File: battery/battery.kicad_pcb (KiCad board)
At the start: 2 copper layers, 73.7 x 63.5 mm, 48 parts, among them J1 batt_1, J2 batt_2, J3 batt_3, J4 batt_4, J5 reed_switch, J6 toPcb+, J7 toPcb-, J8 on_signal, Q1 batt1_sw, Q2 batt2_sw, Q3 batt3_sw, Q4 batt4_sw, Q5 Q_NPN_CBE, U1 LM1117-5.0, U2 LTV-817S

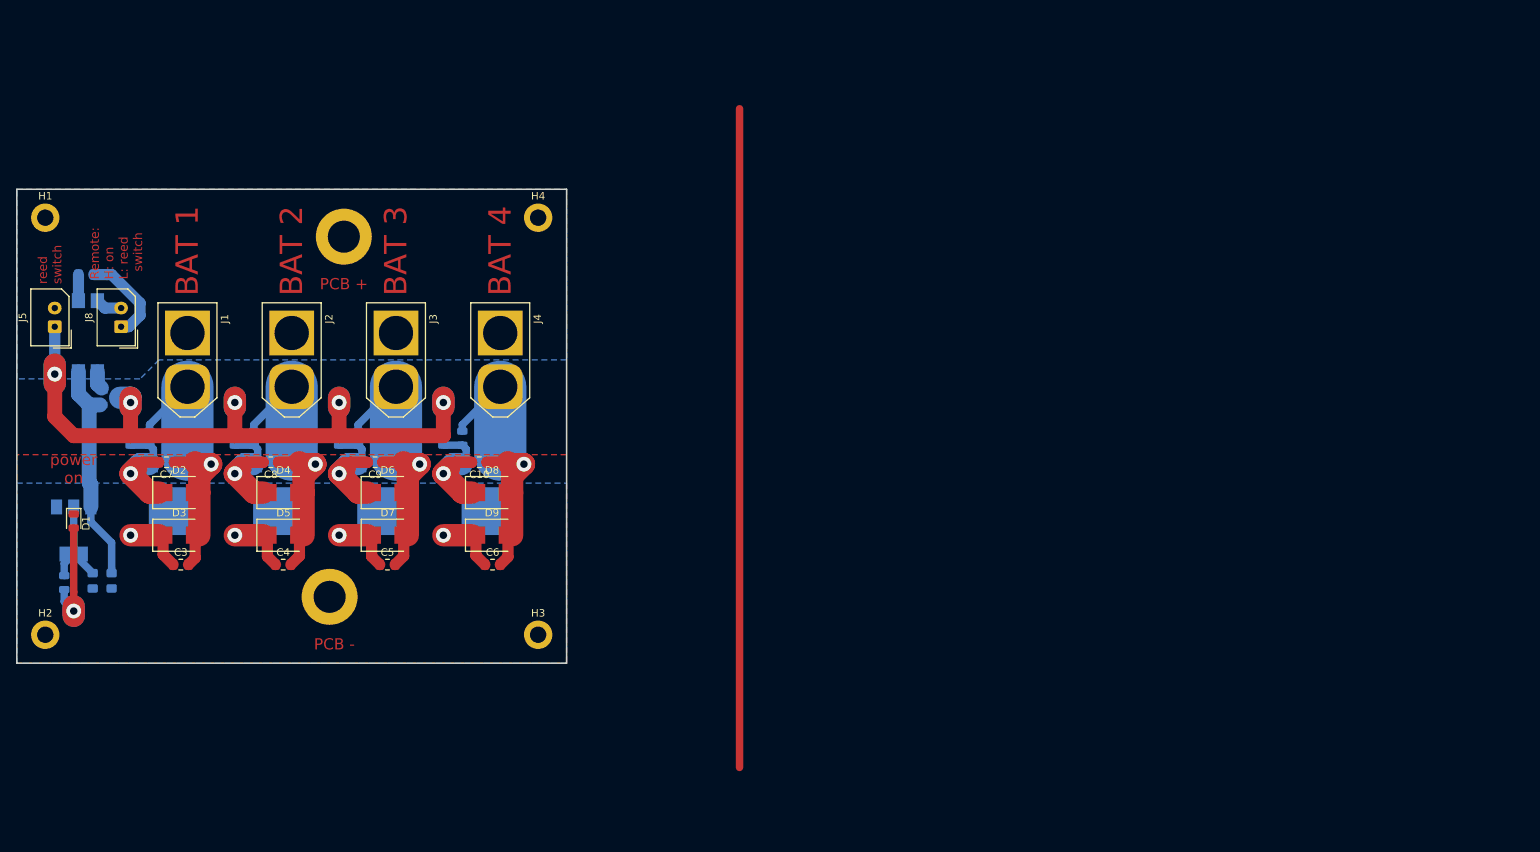
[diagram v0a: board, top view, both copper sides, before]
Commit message: fix
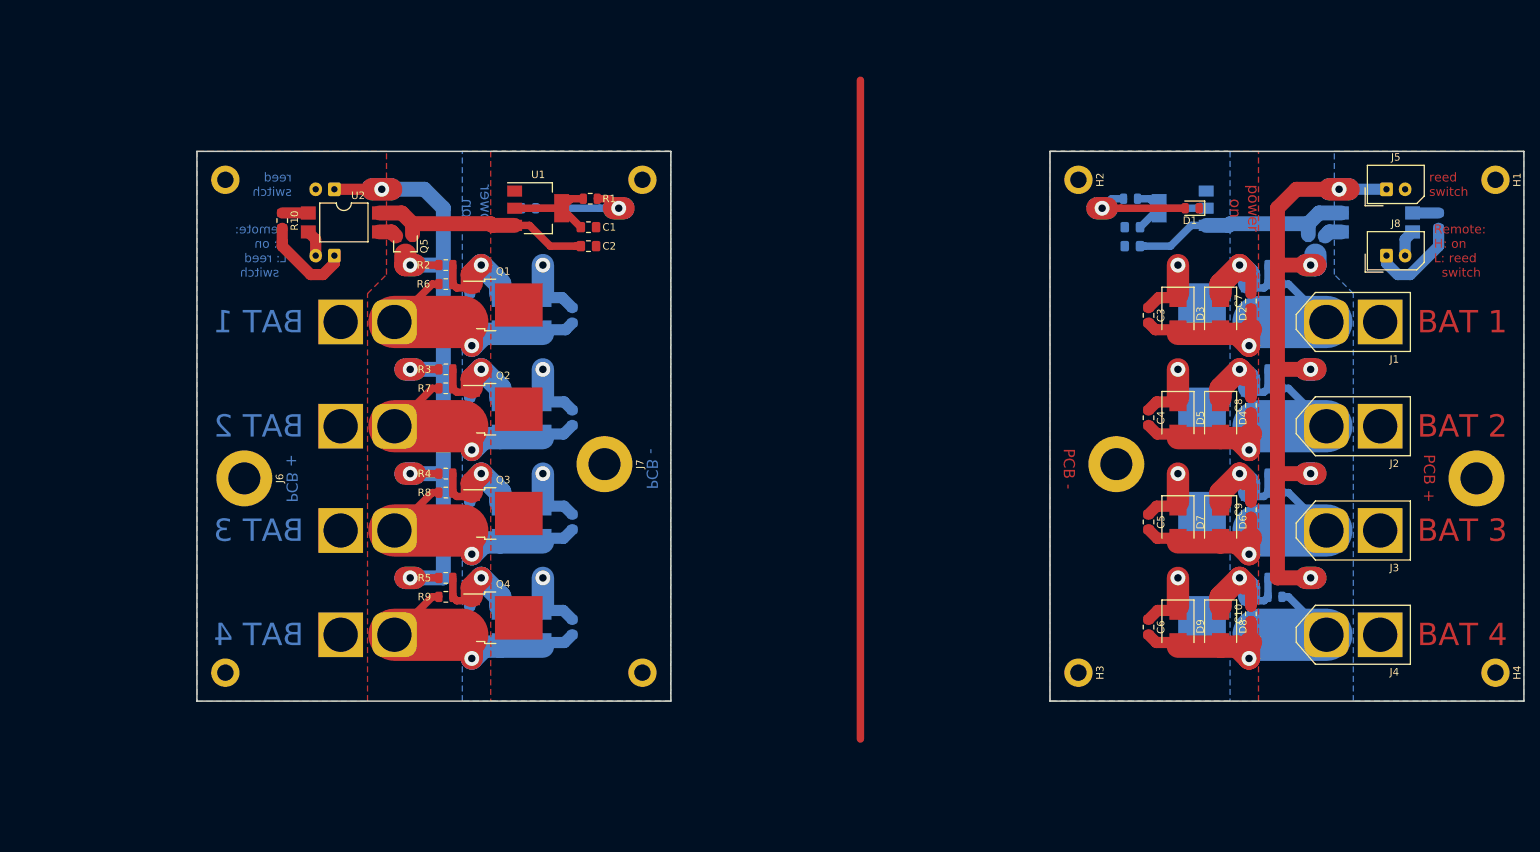
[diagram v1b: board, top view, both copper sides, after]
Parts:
- removed the C1 at (65.4, 116.0)
- removed the C10 at (117.2, 100.1)
- removed the C2 at (67.9, 116.0)
- removed the C3 at (77.2, 113.8)
- removed the C4 at (90.9, 113.8)
- removed the C5 at (104.9, 113.8)
- removed the C6 at (119.0, 113.8)
- removed the C7 at (75.3, 100.1)
- removed the C8 at (89.3, 100.1)
- removed the C9 at (103.2, 100.1)
- removed the D1 at (62.9, 108.0)
- removed the D2 at (77.0, 104.1)
- removed the D3 at (77.0, 109.9)
- removed the D4 at (91.0, 104.1)
- removed the D5 at (91.0, 109.9)
- removed the D6 at (104.9, 104.1)
- removed the D7 at (104.9, 109.9)
- removed the D8 at (118.9, 104.1)
- removed the D9 at (118.9, 109.9)
- removed the H1 at (59.1, 67.3)
- removed the H2 at (59.1, 123.2)
- removed the H3 at (125.1, 123.2)
- removed the H4 at (125.1, 67.3)
- removed the J1 at (78.1, 86.4)
- removed the J2 at (92.1, 86.4)
- removed the J3 at (106.0, 86.4)
- removed the J4 at (120.0, 86.4)
- removed the J5 at (60.3, 81.9)
- removed the J6 at (99.1, 69.8)
- removed the J7 at (97.2, 118.1)
- removed the J8 at (69.2, 81.9)
- removed the Q1 at (75.8, 104.5)
- removed the Q2 at (89.8, 104.5)
- removed the Q3 at (103.8, 104.5)
- removed the Q4 at (117.7, 104.5)
- removed the Q5 at (67.9, 91.4)
- removed the R1 at (61.6, 116.2)
- removed the R10 at (64.5, 74.9)
- removed the R2 at (70.5, 96.9)
- removed the R3 at (84.5, 96.9)
- removed the R4 at (98.4, 96.9)
- removed the R5 at (112.4, 96.9)
- removed the R6 at (73.0, 96.9)
- removed the R7 at (87.0, 96.9)
- removed the R8 at (101.0, 96.9)
- removed the R9 at (114.9, 96.9)
- removed the U1 at (62.9, 109.2)
- removed the U2 at (64.8, 83.2)
- added C1: C_Small, Capacitor_SMD:C_0805_2012Metric_Pad1.15x1.40mm_HandSolder, B.Cu at (204.7, 68.6)
- added C1: C_Small, Capacitor_SMD:C_0805_2012Metric_Pad1.15x1.40mm_HandSolder, F.Cu at (131.8, 68.6)
- added C10: 100n, Capacitor_SMD:C_0805_2012Metric_Pad1.15x1.40mm_HandSolder, F.Cu at (220.6, 120.4)
- added C10: 100n, Capacitor_SMD:C_0805_2012Metric_Pad1.15x1.40mm_HandSolder, B.Cu at (116.0, 120.4)
- added C2: C_Small, Capacitor_SMD:C_0805_2012Metric_Pad1.15x1.40mm_HandSolder, B.Cu at (204.7, 71.1)
- added C2: C_Small, Capacitor_SMD:C_0805_2012Metric_Pad1.15x1.40mm_HandSolder, F.Cu at (131.8, 71.1)
- added C3: 10uF, Capacitor_SMD:C_0805_2012Metric_Pad1.15x1.40mm_HandSolder, F.Cu at (206.9, 80.4)
- added C3: 10uF, Capacitor_SMD:C_0805_2012Metric_Pad1.15x1.40mm_HandSolder, B.Cu at (129.7, 80.4)
- added C4: 10uF, Capacitor_SMD:C_0805_2012Metric_Pad1.15x1.40mm_HandSolder, F.Cu at (206.9, 94.1)
- added C4: 10uF, Capacitor_SMD:C_0805_2012Metric_Pad1.15x1.40mm_HandSolder, B.Cu at (129.7, 94.1)
- added C5: 10uF, Capacitor_SMD:C_0805_2012Metric_Pad1.15x1.40mm_HandSolder, F.Cu at (206.9, 108.1)
- added C5: 10uF, Capacitor_SMD:C_0805_2012Metric_Pad1.15x1.40mm_HandSolder, B.Cu at (129.7, 108.1)
- added C6: 10uF, Capacitor_SMD:C_0805_2012Metric_Pad1.15x1.40mm_HandSolder, F.Cu at (206.9, 122.2)
- added C6: 10uF, Capacitor_SMD:C_0805_2012Metric_Pad1.15x1.40mm_HandSolder, B.Cu at (129.7, 122.2)
- added C7: 100n, Capacitor_SMD:C_0805_2012Metric_Pad1.15x1.40mm_HandSolder, F.Cu at (220.6, 78.5)
- added C7: 100n, Capacitor_SMD:C_0805_2012Metric_Pad1.15x1.40mm_HandSolder, B.Cu at (116.0, 78.5)
- added C8: 100n, Capacitor_SMD:C_0805_2012Metric_Pad1.15x1.40mm_HandSolder, F.Cu at (220.6, 92.4)
- added C8: 100n, Capacitor_SMD:C_0805_2012Metric_Pad1.15x1.40mm_HandSolder, B.Cu at (116.0, 92.4)
- added C9: 100n, Capacitor_SMD:C_0805_2012Metric_Pad1.15x1.40mm_HandSolder, F.Cu at (220.6, 106.4)
- added C9: 100n, Capacitor_SMD:C_0805_2012Metric_Pad1.15x1.40mm_HandSolder, B.Cu at (116.0, 106.4)
- added D1: power_ok, LED_SMD:LED_0805_2012Metric, F.Cu at (212.7, 66.0)
- added D1: power_ok, LED_SMD:LED_0805_2012Metric, B.Cu at (123.8, 66.0)
- added D2: D_TVS, Diode_SMD:D_SMB, F.Cu at (216.5, 80.2)
- added D2: D_TVS, Diode_SMD:D_SMB, B.Cu at (120.0, 80.2)
- added D3: D_TVS, Diode_SMD:D_SMB, F.Cu at (210.8, 80.2)
- added D3: D_TVS, Diode_SMD:D_SMB, B.Cu at (125.7, 80.2)
- added D4: D_TVS, Diode_SMD:D_SMB, F.Cu at (216.5, 94.1)
- added D4: D_TVS, Diode_SMD:D_SMB, B.Cu at (120.0, 94.1)
- added D5: D_TVS, Diode_SMD:D_SMB, F.Cu at (210.8, 94.1)
- added D5: D_TVS, Diode_SMD:D_SMB, B.Cu at (125.7, 94.1)
- added D6: D_TVS, Diode_SMD:D_SMB, F.Cu at (216.5, 108.1)
- added D6: D_TVS, Diode_SMD:D_SMB, B.Cu at (120.0, 108.1)
- added D7: D_TVS, Diode_SMD:D_SMB, F.Cu at (210.8, 108.1)
- added D7: D_TVS, Diode_SMD:D_SMB, B.Cu at (125.7, 108.1)
- added D8: D_TVS, Diode_SMD:D_SMB, F.Cu at (216.5, 122.1)
- added D8: D_TVS, Diode_SMD:D_SMB, B.Cu at (120.0, 122.1)
- added D9: D_TVS, Diode_SMD:D_SMB, F.Cu at (210.8, 122.1)
- added D9: D_TVS, Diode_SMD:D_SMB, B.Cu at (125.7, 122.1)
- added H1: mnt, MountingHole:MountingHole_2.2mm_M2_DIN965_Pad, F.Cu at (253.4, 62.2)
- added H1: mnt, MountingHole:MountingHole_2.2mm_M2_DIN965_Pad, B.Cu at (83.2, 62.2)
- added H2: mnt, MountingHole:MountingHole_2.2mm_M2_DIN965_Pad, F.Cu at (197.5, 62.2)
- added H2: mnt, MountingHole:MountingHole_2.2mm_M2_DIN965_Pad, B.Cu at (139.1, 62.2)
- added H3: mnt, MountingHole:MountingHole_2.2mm_M2_DIN965_Pad, F.Cu at (197.5, 128.3)
- added H3: mnt, MountingHole:MountingHole_2.2mm_M2_DIN965_Pad, B.Cu at (139.1, 128.3)
- added H4: mnt, MountingHole:MountingHole_2.2mm_M2_DIN965_Pad, F.Cu at (253.4, 128.3)
- added H4: mnt, MountingHole:MountingHole_2.2mm_M2_DIN965_Pad, B.Cu at (83.2, 128.3)
- added J1: batt_1, power_connectors:XT60UPB-M, F.Cu at (234.3, 81.3)
- added J1: batt_1, power_connectors:XT60UPB-M, B.Cu at (102.2, 81.3)
- added J2: batt_2, power_connectors:XT60UPB-M, F.Cu at (234.3, 95.2)
- added J2: batt_2, power_connectors:XT60UPB-M, B.Cu at (102.2, 95.2)
- added J3: batt_3, power_connectors:XT60UPB-M, F.Cu at (234.3, 109.2)
- added J3: batt_3, power_connectors:XT60UPB-M, B.Cu at (102.2, 109.2)
- added J4: batt_4, power_connectors:XT60UPB-M, F.Cu at (234.3, 123.2)
- added J4: batt_4, power_connectors:XT60UPB-M, B.Cu at (102.2, 123.2)
- added J5: reed_switch, Connector_Molex:Molex_SPOX_5267-02A_1x02_P2.50mm_Vertical, F.Cu at (238.8, 63.5)
- added J5: reed_switch, Connector_Molex:Molex_SPOX_5267-02A_1x02_P2.50mm_Vertical, B.Cu at (97.8, 63.5)
- added J6: toPcb+, MountingHole:MountingHole_4.3mm_M4_DIN965_Pad, B.Cu at (250.8, 102.2)
- added J6: toPcb+, MountingHole:MountingHole_4.3mm_M4_DIN965_Pad, F.Cu at (85.7, 102.2)
- added J7: toPcb-, MountingHole:MountingHole_4.3mm_M4_DIN965_Pad, B.Cu at (202.6, 100.3)
- added J7: toPcb-, MountingHole:MountingHole_4.3mm_M4_DIN965_Pad, F.Cu at (134.0, 100.3)
- added J8: on_signal, Connector_Molex:Molex_SPOX_5267-02A_1x02_P2.50mm_Vertical, F.Cu at (238.8, 72.4)
- added J8: on_signal, Connector_Molex:Molex_SPOX_5267-02A_1x02_P2.50mm_Vertical, B.Cu at (97.8, 72.4)
- added Q1: batt1_sw, Package_TO_SOT_SMD:TO-252-2, B.Cu at (216.1, 79.0)
- added Q1: batt1_sw, Package_TO_SOT_SMD:TO-252-2, F.Cu at (120.4, 79.0)
- added Q2: batt2_sw, Package_TO_SOT_SMD:TO-252-2, B.Cu at (216.1, 93.0)
- added Q2: batt2_sw, Package_TO_SOT_SMD:TO-252-2, F.Cu at (120.4, 93.0)
- added Q3: batt3_sw, Package_TO_SOT_SMD:TO-252-2, B.Cu at (216.1, 106.9)
- added Q3: batt3_sw, Package_TO_SOT_SMD:TO-252-2, F.Cu at (120.4, 106.9)
- added Q4: batt4_sw, Package_TO_SOT_SMD:TO-252-2, B.Cu at (216.1, 120.9)
- added Q4: batt4_sw, Package_TO_SOT_SMD:TO-252-2, F.Cu at (120.4, 120.9)
- added Q5: Q_NPN_CBE, Package_TO_SOT_SMD:SOT-23, B.Cu at (229.2, 71.1)
- added Q5: Q_NPN_CBE, Package_TO_SOT_SMD:SOT-23, F.Cu at (107.3, 71.1)
- added R1: 400, Resistor_SMD:R_0805_2012Metric, B.Cu at (204.5, 64.8)
- added R1: 400, Resistor_SMD:R_0805_2012Metric, F.Cu at (132.1, 64.8)
- added R10: R, Resistor_SMD:R_0805_2012Metric_Pad1.15x1.40mm_HandSolder, B.Cu at (245.7, 67.7)
- added R10: R, Resistor_SMD:R_0805_2012Metric_Pad1.15x1.40mm_HandSolder, F.Cu at (90.8, 67.7)
- added R2: 100, Resistor_SMD:R_0805_2012Metric, B.Cu at (223.8, 73.7)
- added R2: 100, Resistor_SMD:R_0805_2012Metric, F.Cu at (112.7, 73.7)
- added R3: 100, Resistor_SMD:R_0805_2012Metric, B.Cu at (223.8, 87.6)
- added R3: 100, Resistor_SMD:R_0805_2012Metric, F.Cu at (112.7, 87.6)
- added R4: 100, Resistor_SMD:R_0805_2012Metric, B.Cu at (223.8, 101.6)
- added R4: 100, Resistor_SMD:R_0805_2012Metric, F.Cu at (112.7, 101.6)
- added R5: 100, Resistor_SMD:R_0805_2012Metric, B.Cu at (223.8, 115.6)
- added R5: 100, Resistor_SMD:R_0805_2012Metric, F.Cu at (112.7, 115.6)
- added R6: 47k, Resistor_SMD:R_0805_2012Metric, B.Cu at (223.8, 76.2)
- added R6: 47k, Resistor_SMD:R_0805_2012Metric, F.Cu at (112.7, 76.2)
- added R7: 47k, Resistor_SMD:R_0805_2012Metric, B.Cu at (223.8, 90.2)
- added R7: 47k, Resistor_SMD:R_0805_2012Metric, F.Cu at (112.7, 90.2)
- added R8: 47k, Resistor_SMD:R_0805_2012Metric, B.Cu at (223.8, 104.1)
- added R8: 47k, Resistor_SMD:R_0805_2012Metric, F.Cu at (112.7, 104.1)
- added R9: 47k, Resistor_SMD:R_0805_2012Metric, B.Cu at (223.8, 118.1)
- added R9: 47k, Resistor_SMD:R_0805_2012Metric, F.Cu at (112.7, 118.1)
- added U1: LM1117-5.0, Package_TO_SOT_SMD:SOT-223-3_TabPin2, B.Cu at (211.5, 66.0)
- added U1: LM1117-5.0, Package_TO_SOT_SMD:SOT-223-3_TabPin2, F.Cu at (125.1, 66.0)
- added U2: LTV-817S, Package_DIP:SMDIP-4_W9.53mm, B.Cu at (237.5, 67.9)
- added U2: LTV-817S, Package_DIP:SMDIP-4_W9.53mm, F.Cu at (99.1, 67.9)
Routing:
- net Net-(J5-Pad1): track 115.6 -> 231.2 mm, vias 5 -> 10
- net Net-(C5-Pad2): track 43.8 -> 87.6 mm, vias 1 -> 2
- net Net-(C4-Pad2): track 43.8 -> 87.6 mm, vias 1 -> 2
- net Net-(C10-Pad1): track 43.7 -> 87.5 mm, vias 1 -> 2
- net Net-(C3-Pad2): track 40.4 -> 80.8 mm, vias 1 -> 2
- net gnd: track 33.0 -> 65.9 mm, vias 4 -> 8
- net Vin: track 30.3 -> 60.6 mm
- net Net-(C8-Pad2): track 21.4 -> 42.7 mm, vias 1 -> 2
- net Net-(C9-Pad2): track 20.9 -> 41.7 mm, vias 1 -> 2
- net Net-(C10-Pad2): track 20.9 -> 41.7 mm, vias 1 -> 2
- net Net-(C7-Pad2): track 18.6 -> 37.2 mm, vias 1 -> 2
- net Net-(D1-Pad2): track 17.1 -> 34.1 mm, vias 1 -> 2
- net Net-(C1-Pad1): track 13.3 -> 26.7 mm
- net Net-(J8-Pad1): track 12.6 -> 25.2 mm
- net Net-(J8-Pad2): track 3.59 -> 7.17 mm
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- added copper zone on F.Cu, net Vin
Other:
- board size 73.7 x 63.5 mm -> 177.8 x 73.7 mm

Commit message: new schematic
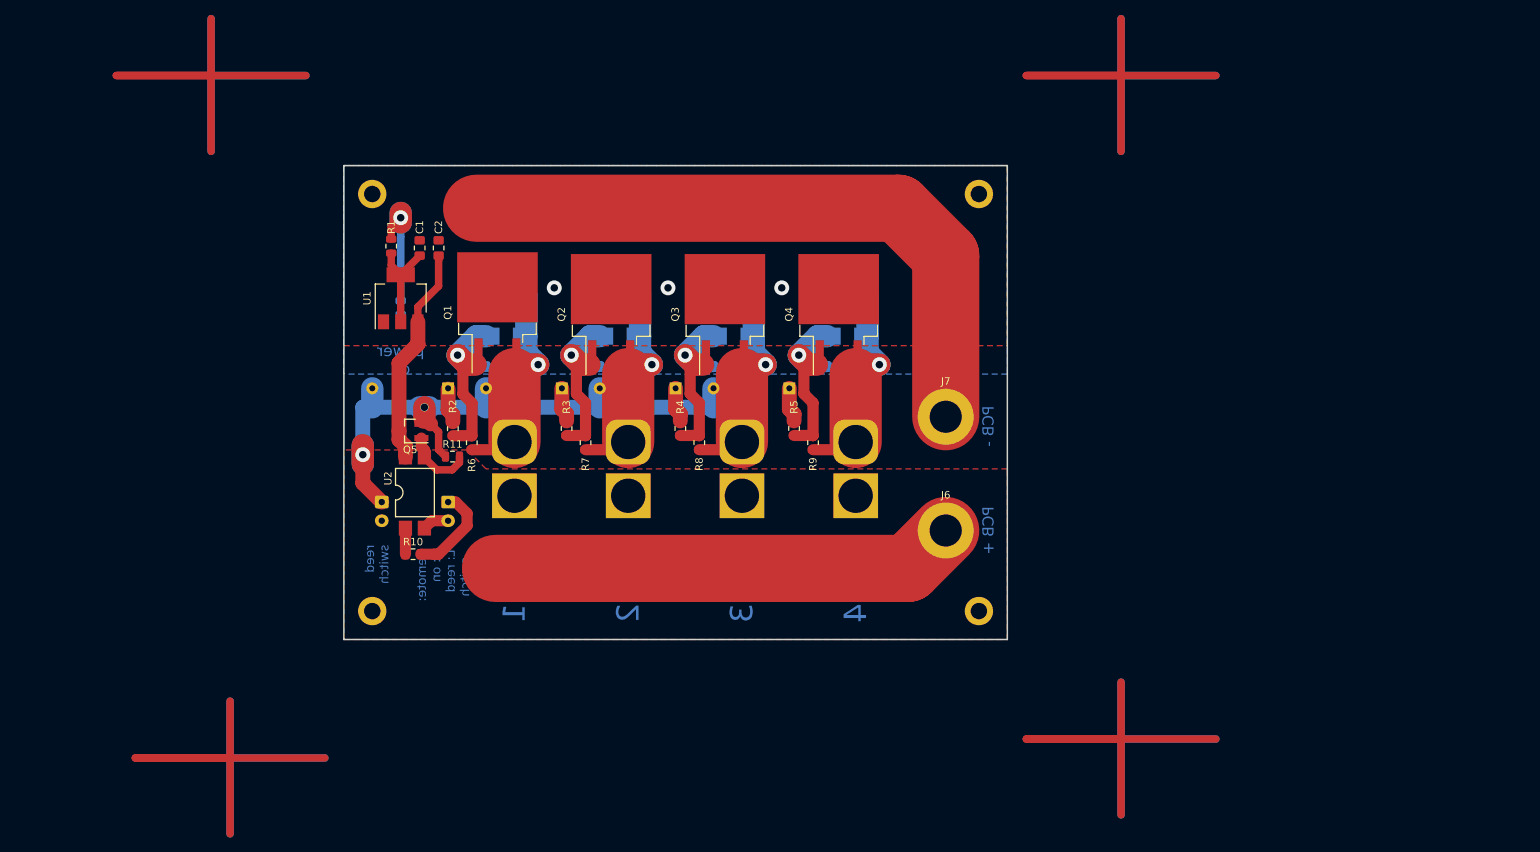
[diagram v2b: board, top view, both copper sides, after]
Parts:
- removed the C1 at (204.7, 68.6)
- removed the C10 at (220.6, 120.4)
- removed the C10 at (116.0, 120.4)
- removed the C2 at (204.7, 71.1)
- removed the C3 at (206.9, 80.4)
- removed the C3 at (129.7, 80.4)
- removed the C4 at (206.9, 94.1)
- removed the C4 at (129.7, 94.1)
- removed the C5 at (206.9, 108.1)
- removed the C5 at (129.7, 108.1)
- removed the C6 at (206.9, 122.2)
- removed the C6 at (129.7, 122.2)
- removed the C7 at (220.6, 78.5)
- removed the C8 at (220.6, 92.4)
- removed the C8 at (116.0, 92.4)
- removed the C9 at (220.6, 106.4)
- removed the C9 at (116.0, 106.4)
- removed the D1 at (212.7, 66.0)
- removed the D2 at (216.5, 80.2)
- removed the D3 at (210.8, 80.2)
- removed the D4 at (216.5, 94.1)
- removed the D4 at (120.0, 94.1)
- removed the D5 at (210.8, 94.1)
- removed the D5 at (125.7, 94.1)
- removed the D6 at (216.5, 108.1)
- removed the D6 at (120.0, 108.1)
- removed the D7 at (210.8, 108.1)
- removed the D7 at (125.7, 108.1)
- removed the D8 at (216.5, 122.1)
- removed the D8 at (120.0, 122.1)
- removed the D9 at (210.8, 122.1)
- removed the D9 at (125.7, 122.1)
- removed the H1 at (253.4, 62.2)
- removed the H2 at (197.5, 62.2)
- removed the H3 at (197.5, 128.3)
- removed the H3 at (139.1, 128.3)
- removed the H4 at (253.4, 128.3)
- removed the J1 at (234.3, 81.3)
- removed the J2 at (234.3, 95.2)
- removed the J2 at (102.2, 95.2)
- removed the J3 at (234.3, 109.2)
- removed the J3 at (102.2, 109.2)
- removed the J4 at (234.3, 123.2)
- removed the J4 at (102.2, 123.2)
- removed the J5 at (238.8, 63.5)
- removed the J6 at (250.8, 102.2)
- removed the J7 at (202.6, 100.3)
- removed the J8 at (238.8, 72.4)
- removed the Q1 at (216.1, 79.0)
- removed the Q1 at (120.4, 79.0)
- removed the Q2 at (216.1, 93.0)
- removed the Q2 at (120.4, 93.0)
- removed the Q3 at (216.1, 106.9)
- removed the Q3 at (120.4, 106.9)
- removed the Q4 at (216.1, 120.9)
- removed the Q4 at (120.4, 120.9)
- removed the Q5 at (229.2, 71.1)
- removed the Q5 at (107.3, 71.1)
- removed the R1 at (204.5, 64.8)
- removed the R10 at (245.7, 67.7)
- removed the R2 at (223.8, 73.7)
- removed the R3 at (223.8, 87.6)
- removed the R4 at (223.8, 101.6)
- removed the R4 at (112.7, 101.6)
- removed the R5 at (223.8, 115.6)
- removed the R5 at (112.7, 115.6)
- removed the R6 at (223.8, 76.2)
- removed the R7 at (223.8, 90.2)
- removed the R7 at (112.7, 90.2)
- removed the R8 at (223.8, 104.1)
- removed the R8 at (112.7, 104.1)
- removed the R9 at (223.8, 118.1)
- removed the R9 at (112.7, 118.1)
- removed the U1 at (211.5, 66.0)
- removed the U2 at (237.5, 67.9)
- added C10: 100n, Capacitor_SMD:C_0805_2012Metric_Pad1.15x1.40mm_HandSolder, B.Cu at (164.8, 87.2)
- added C3: 10uF, Capacitor_SMD:C_1206_3216Metric_Pad1.42x1.75mm_HandSolder, B.Cu at (121.0, 73.5)
- added C4: 10uF, Capacitor_SMD:C_1206_3216Metric_Pad1.42x1.75mm_HandSolder, B.Cu at (136.0, 73.5)
- added C5: 10uF, Capacitor_SMD:C_1206_3216Metric_Pad1.42x1.75mm_HandSolder, B.Cu at (151.3, 73.5)
- added C6: 10uF, Capacitor_SMD:C_1206_3216Metric_Pad1.42x1.75mm_HandSolder, B.Cu at (166.6, 73.5)
- added C8: 100n, Capacitor_SMD:C_0805_2012Metric_Pad1.15x1.40mm_HandSolder, B.Cu at (134.4, 87.2)
- added C9: 100n, Capacitor_SMD:C_0805_2012Metric_Pad1.15x1.40mm_HandSolder, B.Cu at (149.6, 87.2)
- added D10: bat48, Diode_THT:D_DO-35_SOD27_P10.16mm_Horizontal, B.Cu at (113.0, 90.2)
- added D11: bat48, Diode_THT:D_DO-35_SOD27_P10.16mm_Horizontal, B.Cu at (128.3, 90.2)
- added D12: bat48, Diode_THT:D_DO-35_SOD27_P10.16mm_Horizontal, B.Cu at (143.5, 90.2)
- added D13: bat48, Diode_THT:D_DO-35_SOD27_P10.16mm_Horizontal, B.Cu at (158.8, 90.2)
- added D4: D_TVS, Diode_SMD:D_SMB, B.Cu at (136.1, 83.2)
- added D5: D_TVS, Diode_SMD:D_SMB, B.Cu at (136.1, 77.5)
- added D6: D_TVS, Diode_SMD:D_SMB, B.Cu at (151.3, 83.2)
- added D7: D_TVS, Diode_SMD:D_SMB, B.Cu at (151.3, 77.5)
- added D8: D_TVS, Diode_SMD:D_SMB, B.Cu at (166.5, 83.2)
- added D9: D_TVS, Diode_SMD:D_SMB, B.Cu at (166.5, 77.5)
- added H3: mnt, MountingHole:MountingHole_2.2mm_M2_DIN965_Pad, B.Cu at (184.2, 64.1)
- added J2: batt_2, power_connectors:XT60UPB-M, B.Cu at (137.2, 101.0)
- added J3: batt_3, power_connectors:XT60UPB-M, B.Cu at (152.4, 101.0)
- added J4: batt_4, power_connectors:XT60UPB-M, B.Cu at (167.6, 101.0)
- added Q1: batt1_sw, Package_TO_SOT_SMD:TO-263-2, F.Cu at (119.6, 80.0)
- added Q2: batt2_sw, Package_TO_SOT_SMD:TO-263-2, F.Cu at (134.9, 80.3)
- added Q3: batt3_sw, Package_TO_SOT_SMD:TO-263-2, F.Cu at (150.1, 80.3)
- added Q4: batt4_sw, Package_TO_SOT_SMD:TO-263-2, F.Cu at (165.4, 80.3)
- added Q5: BC817-25, Package_TO_SOT_SMD:SOT-23_Handsoldering, F.Cu at (108.0, 95.9)
- added R11: 10k, Resistor_SMD:R_0805_2012Metric, F.Cu at (113.6, 99.3)
- added R4: 100, Resistor_SMD:R_0805_2012Metric, F.Cu at (144.1, 95.6)
- added R5: 100, Resistor_SMD:R_0805_2012Metric, F.Cu at (159.4, 95.6)
- added R7: 47k, Resistor_SMD:R_0805_2012Metric, F.Cu at (131.4, 97.5)
- added R8: 47k, Resistor_SMD:R_0805_2012Metric, F.Cu at (146.7, 97.5)
- added R9: 47k, Resistor_SMD:R_0805_2012Metric, F.Cu at (161.9, 97.5)
- R10: value R -> 680
- moved H4 101.3 mm to (184.2, 120.0), turned to 0 degrees
- moved J6 94.2 mm to (179.7, 109.2), turned to 0 degrees
- moved H1 61.0 mm to (102.9, 120.0), turned to 0 degrees
- moved R10 48.0 mm to (108.3, 112.4), turned to 0 degrees
- moved J7 46.2 mm to (179.7, 94.0), turned to 0 degrees
- moved J5 42.4 mm to (104.1, 105.4), turned to 270 degrees
- moved U2 37.4 mm to (108.6, 104.1), turned to 90 degrees
- moved J8 36.4 mm to (113.0, 105.4), turned to 270 degrees
- moved H2 36.2 mm to (102.9, 64.1), turned to 0 degrees
- moved J1 27.8 mm to (121.9, 101.0), turned to 90 degrees
- moved R1 27.4 mm to (105.4, 71.1), turned to 270 degrees
- moved C1 22.8 mm to (109.2, 71.4), turned to 90 degrees
- moved U1 22.0 mm to (106.7, 78.1), turned to 90 degrees
- moved R2 21.9 mm to (113.7, 95.6), turned to 90 degrees
- moved D1 21.7 mm to (106.7, 79.4), turned to 90 degrees
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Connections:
- J5 pad 1: Net-(J5-Pad1) -> Net-(D10-Pad2)
- R2 pad 2: Net-(J5-Pad1) -> Net-(D10-Pad1)
- R3 pad 2: Net-(J5-Pad1) -> Net-(D11-Pad1)
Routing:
- net (no net): track 88.3 -> 396.2 mm
- net Net-(J5-Pad1): track 231.2 -> 0.00 mm, vias 10 -> 0
- net Net-(D10-Pad2): track 0.00 -> 86.3 mm, vias 0 -> 2
- net Net-(C5-Pad2): track 87.6 -> 41.7 mm, vias 2 -> 1
- net Net-(C4-Pad2): track 87.6 -> 41.7 mm, vias 2 -> 1
- net Net-(C10-Pad1): track 87.5 -> 41.6 mm, vias 2 -> 1
- net Net-(C3-Pad2): track 80.8 -> 40.7 mm, vias 2 -> 1
- net Vin: track 60.6 -> 92.3 mm
- net gnd: track 65.9 -> 87.1 mm, vias 8 -> 3
- net Net-(D1-Pad2): track 34.1 -> 17.1 mm, vias 2 -> 1
- net Net-(C8-Pad2): track 42.7 -> 28.1 mm, vias 2 -> 1
- net Net-(C10-Pad2): track 41.7 -> 27.6 mm, vias 2 -> 1
- net Net-(C1-Pad1): track 26.7 -> 13.3 mm
- net Net-(C9-Pad2): track 41.7 -> 28.4 mm, vias 2 -> 1
- net Net-(J8-Pad1): track 25.2 -> 12.6 mm
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- removed copper zone on B.Cu, net Vin
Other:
- board size 177.8 x 73.7 mm -> 88.9 x 63.5 mm
